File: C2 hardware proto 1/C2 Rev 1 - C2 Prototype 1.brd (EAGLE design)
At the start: 101.6 x 101.6 mm, 28 parts

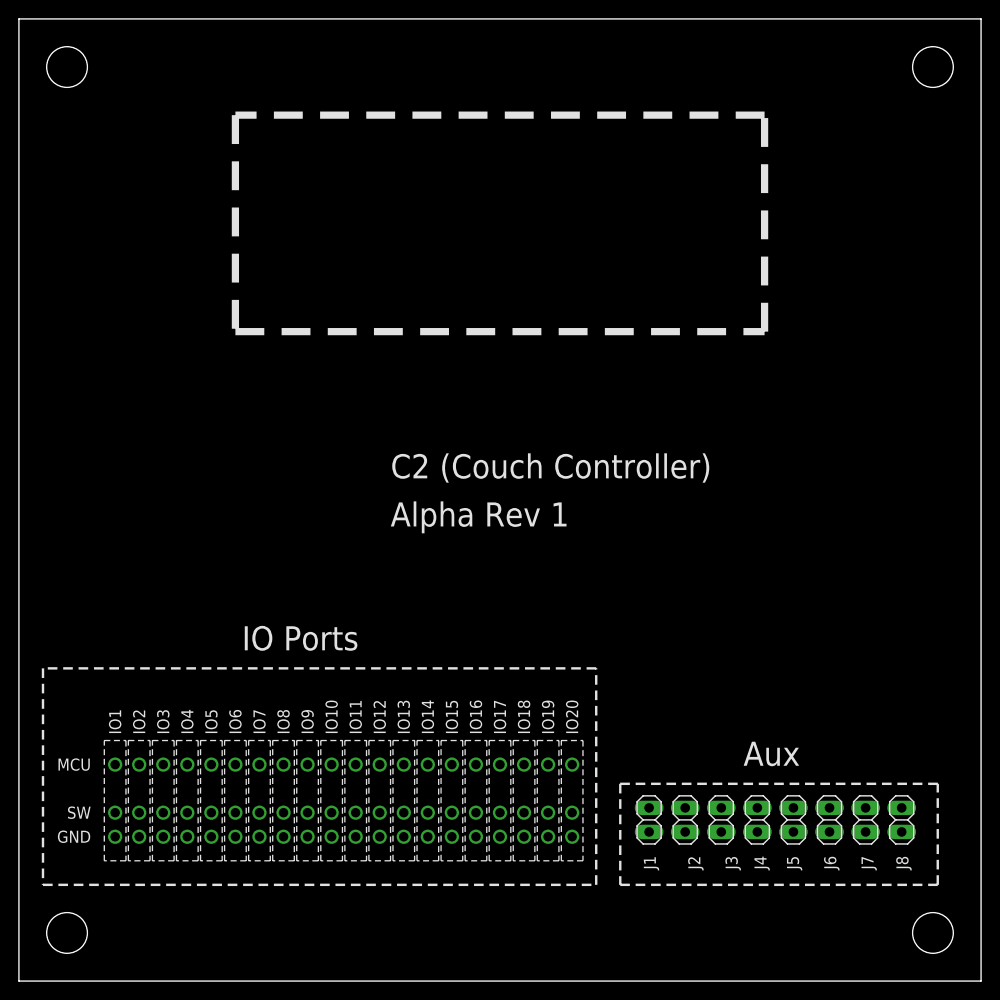
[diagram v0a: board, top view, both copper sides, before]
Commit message: updates
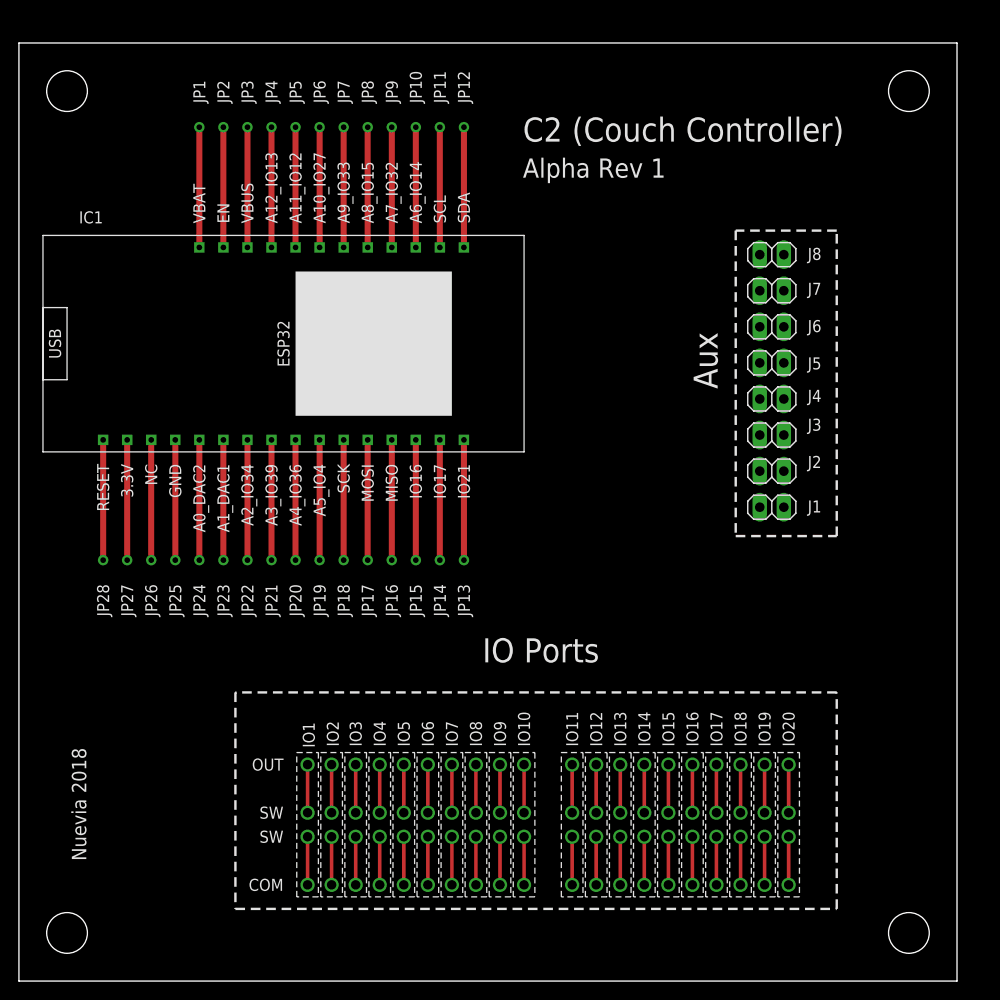
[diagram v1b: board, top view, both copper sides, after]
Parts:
- added IC1: FEATHER-ESP32, VCO-Eagle_parts:ESP32_FEATHER
- added JP1, JP10, JP11, JP12, JP13, JP14, JP15, JP16, JP17, JP18, JP19, JP2, JP20, JP21, JP22, JP23, JP24, JP25, JP26, JP27, JP28, JP3, JP4, JP5, JP6, JP7, JP8, JP9: PROTO_VIA_COMPACT, VanEagleLib:PROTO_VIA
- moved J8 61.2 mm to (79.5, 76.7), turned to 180 degrees
- moved J7 56.8 mm to (79.5, 72.9), turned to 180 degrees
- moved J6 52.4 mm to (79.5, 69.1), turned to 180 degrees
- moved J5 48.3 mm to (79.5, 65.3), turned to 180 degrees
- moved J4 44.5 mm to (79.5, 61.5), turned to 180 degrees
- moved J3 41.0 mm to (79.5, 57.7), turned to 180 degrees
- moved J2 37.9 mm to (79.5, 53.8), turned to 180 degrees
- moved J1 35.5 mm to (79.5, 50.0), turned to 180 degrees
- moved IO14 23.4 mm to (66.0, 10.2)
- moved IO16 23.4 mm to (71.1, 10.2)
- moved IO11 23.4 mm to (58.4, 10.2)
- moved IO12 23.4 mm to (61.0, 10.2)
- moved IO13 23.4 mm to (63.5, 10.2)
- moved IO15 23.4 mm to (68.6, 10.2)
- moved IO17 23.4 mm to (73.7, 10.2)
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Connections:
- removed net GND: IO1.1, IO10.1, IO11.1, IO12.1, IO13.1, IO14.1, IO15.1, IO16.1, IO17.1, IO18.1, IO19.1, IO2.1, IO20.1, IO3.1, IO4.1, IO5.1, IO6.1, IO7.1, IO8.1, IO9.1
- new net COM: IO1.1, IO1.2, IO10.1, IO10.2, IO11.1, IO11.2, IO12.1, IO12.2, IO13.1, IO13.2, IO14.1, IO14.2, IO15.1, IO15.2, IO16.1, IO16.2, IO17.1, IO17.2, IO18.1, IO18.2, IO19.1, IO19.2, IO2.1, IO2.2, IO20.1, IO20.2, IO3.1, IO3.2, IO4.1, IO4.2, IO5.1, IO5.2, IO6.1, IO6.2, IO7.1, IO7.2, IO8.1, IO8.2, IO9.1, IO9.2
- new net N$1: IC1.RESET, JP28.1
- new net N$10: IC1.A5_IO4, JP19.1
- new net N$11: IC1.SCK, JP18.1
- new net N$12: IC1.MOSI, JP17.1
- new net N$13: IC1.MISO, JP16.1
- new net N$14: IC1.IO16, JP15.1
- new net N$15: IC1.IO17, JP14.1
- new net N$16: IC1.IO21, JP13.1
- new net N$17: IC1.SDA, JP12.1
- new net N$18: IC1.SCL, JP11.1
- new net N$19: IC1.A6_IO14, JP10.1
- new net N$2: IC1.3.3V, JP27.1
- new net N$20: IC1.A7_IO32, JP9.1
- new net N$21: IC1.A8_IO15, JP8.1
- new net N$22: IC1.A9_IO33, JP7.1
- new net N$23: IC1.A10_IO27, JP6.1
- new net N$24: IC1.A11_IO12, JP5.1
- new net N$25: IC1.A12_IO13, JP4.1
- new net N$26: IC1.VBUS, JP3.1
- new net N$27: IC1.EN, JP2.1
- new net N$28: IC1.VBAT, JP1.1
- new net N$3: IC1.NC, JP26.1
- new net N$4: IC1.GND, JP25.1
- new net N$5: IC1.A0_DAC2, JP24.1
- new net N$6: IC1.A1_DAC1, JP23.1
- new net N$7: IC1.A2_IO34, JP22.1
- new net N$8: IC1.A3_IO39, JP21.1
- new net N$9: IC1.A4_IO36, JP20.1
- net D1: now also IO1.4; no longer IO1.2
- net D10: now also IO10.4; no longer IO10.2
- net D11: now also IO11.4; no longer IO11.2
- net D12: now also IO12.4; no longer IO12.2
- net D13: now also IO13.4; no longer IO13.2
- net D14: now also IO14.4; no longer IO14.2
- net D15: now also IO15.4; no longer IO15.2
- net D16: now also IO16.4; no longer IO16.2
- net D17: now also IO17.4; no longer IO17.2
- net D18: now also IO18.4; no longer IO18.2
- net D19: now also IO19.4; no longer IO19.2
- net D2: now also IO2.4; no longer IO2.2
- net D20: now also IO20.4; no longer IO20.2
- net D3: now also IO3.4; no longer IO3.2
- net D4: now also IO4.4; no longer IO4.2
- net D5: now also IO5.4; no longer IO5.2
- net D6: now also IO6.4; no longer IO6.2
- net D7: now also IO7.4; no longer IO7.2
- net D8: now also IO8.4; no longer IO8.2
- net D9: now also IO9.4; no longer IO9.2
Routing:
- net COM: track 0.00 -> 101.6 mm
- net N$28: track 0.00 -> 12.7 mm
- net N$27: track 0.00 -> 12.7 mm
- net N$26: track 0.00 -> 12.7 mm
- net N$25: track 0.00 -> 12.7 mm
- net N$24: track 0.00 -> 12.7 mm
- net N$23: track 0.00 -> 12.7 mm
- net N$22: track 0.00 -> 12.7 mm
- net N$21: track 0.00 -> 12.7 mm
- net N$20: track 0.00 -> 12.7 mm
- net N$19: track 0.00 -> 12.7 mm
- net N$18: track 0.00 -> 12.7 mm
- net N$17: track 0.00 -> 12.7 mm
- net N$9: track 0.00 -> 12.7 mm
- net N$8: track 0.00 -> 12.7 mm
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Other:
- board size 101.6 x 101.6 mm -> 99.1 x 99.1 mm
- board text added: "COM"
- board text added: "Nuevia 2018"
- board text added: "OUT"
- board text removed: "GND"
- board text removed: "MCU"
